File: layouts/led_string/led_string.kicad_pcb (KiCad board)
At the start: 2 copper layers, 6 parts

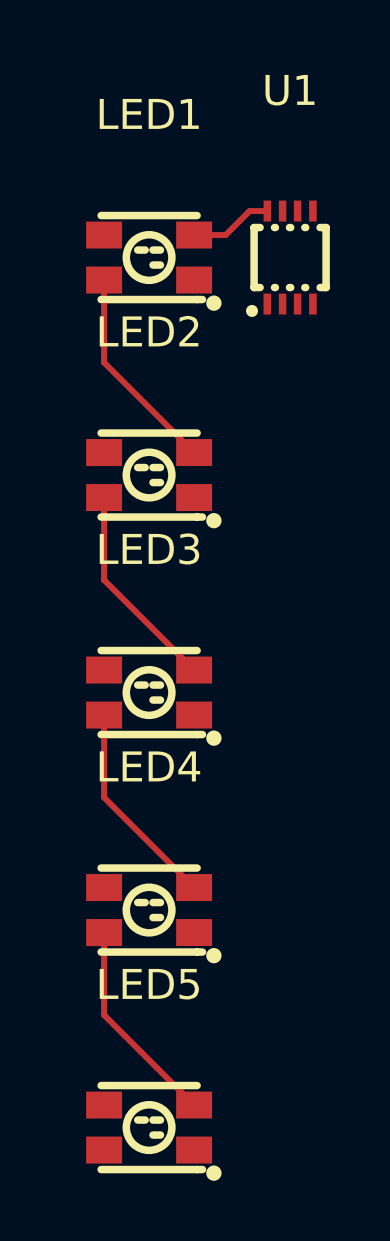
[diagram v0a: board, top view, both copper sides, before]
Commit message: Update layout
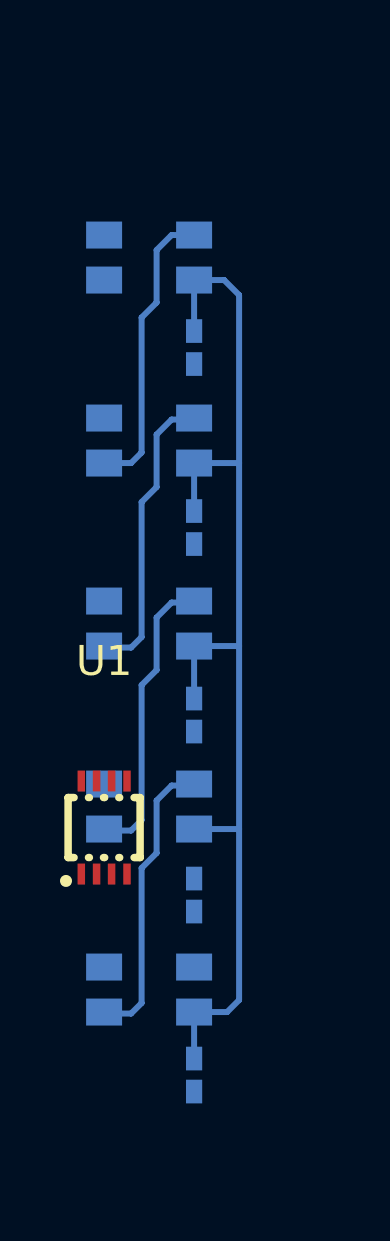
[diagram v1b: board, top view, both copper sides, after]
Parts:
- added C1: 100nF ±10% 16V X7R, atopile:C0402-b3ef17, B.Cu at (1.50, 3.00)
- added C2: 100nF ±10% 16V X7R, atopile:C0402-b3ef17, B.Cu at (1.50, 9.00)
- added C3: 100nF ±10% 16V X7R, atopile:C0402-b3ef17, B.Cu at (1.50, 15.2)
- added C4: 100nF ±10% 16V X7R, atopile:C0402-b3ef17, B.Cu at (1.50, 21.2)
- added C5: 100nF ±10% 16V X7R, atopile:C0402-b3ef17, B.Cu at (1.50, 27.2)
- LED1, LED2, LED3, LED4, LED5: moved to B.Cu
- moved U1 20.0 mm to (-1.50, 19.0)
- moved LED5 4.60 mm to (0.00, 24.4), turned to 180 degrees
- moved LED4 3.45 mm to (0.00, 18.3), turned to 180 degrees
- moved LED3 2.30 mm to (0.00, 12.2), turned to 180 degrees
- moved LED2 1.15 mm to (0.00, 6.10), turned to 180 degrees
- turned LED1 to 180 degrees
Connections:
- LED1 pad 2: line-3 -> line-5
- LED2 pad 4: line-5 -> line-4
- LED3 pad 2: line-5 -> line-4
- LED4 pad 4: line-4 -> line-1
- LED5 pad 2: line-4 -> line-1
- U1 pad 1: runtime_anon[0]-line-1 -> runtime_anon[0]-line
- U1 pad 4: runtime_anon[0]-line -> runtime_anon[0]-line-1
- U1 pad 5: line-1 -> line-3
- U1 pad 8: line-3 -> line-5
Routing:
- net hv-1: track 0.00 -> 38.0 mm
- net line-1: track 0.00 -> 9.81 mm
- net line-5: track 6.99 -> 0.00 mm
- net line-2: track 6.99 -> 9.81 mm
- net line-4: track 6.99 -> 9.81 mm
- net line: track 6.99 -> 9.81 mm
- net line-3: track 2.77 -> 0.00 mm
